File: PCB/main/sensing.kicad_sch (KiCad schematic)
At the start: 4 parts, among them U4 TO-92_Temperature_Sensor, U5 C94049_Barometer

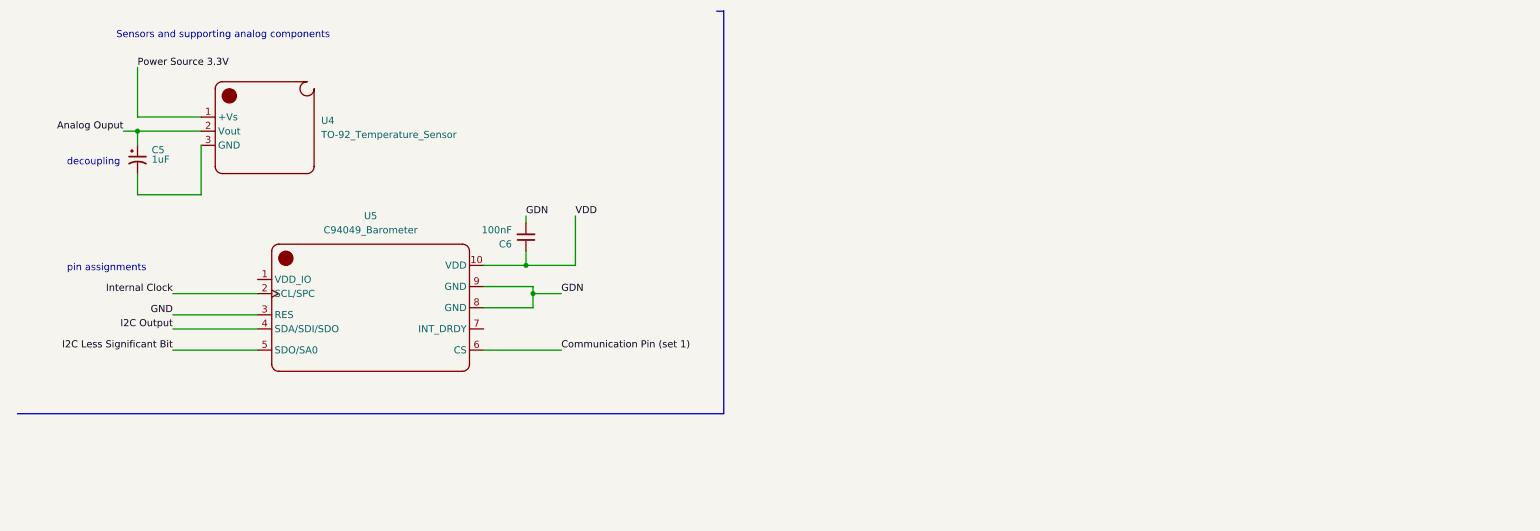
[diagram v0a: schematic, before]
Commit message: Finished initial design
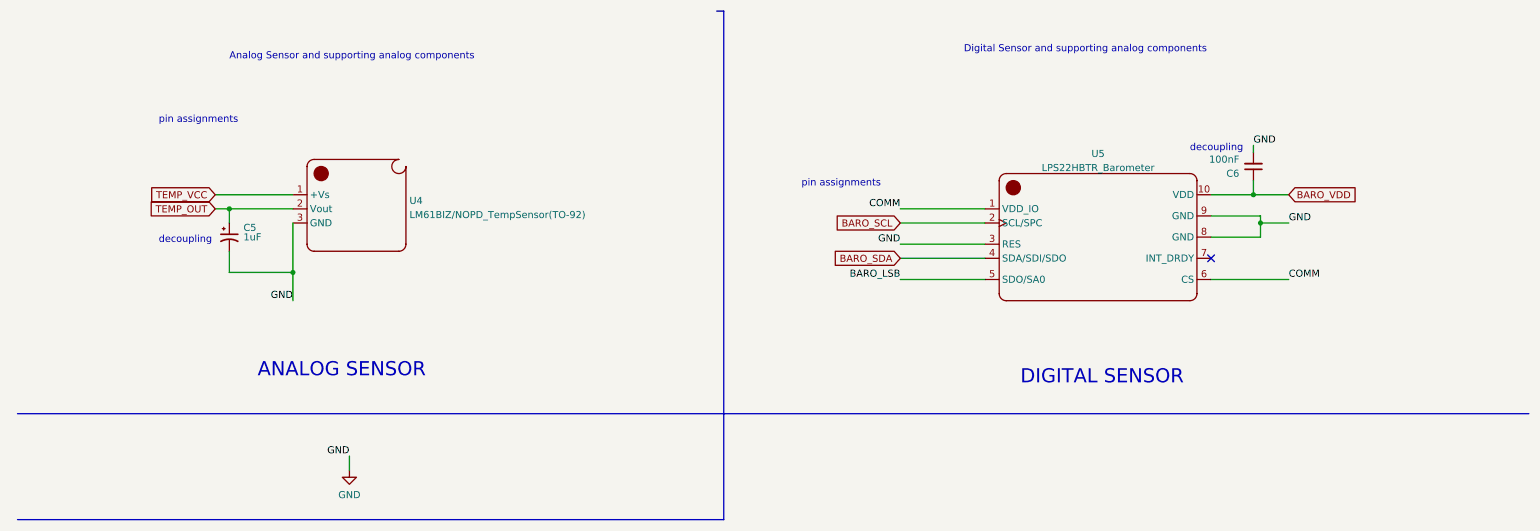
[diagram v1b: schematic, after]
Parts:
- U4: value TO-92_Temperature_Sensor -> LM61BIZ/NOPD_TempSensor(TO-92)
- U5: value C94049_Barometer -> LPS22HBTR_Barometer
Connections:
- net Communication Pin (set 1) is gone; now on net COMM: U5.6 (CS)
- net GDN is gone; now on net GND: C6.2, U5.8 (GND), U5.9 (GND)
- net GND: now also C5.2, U4.3 (GND)
- net COMM: now reaches U5.1 (VDD_IO)
- net Analog Ouput renamed TEMP_OUT
- net I2C Less Significant Bit renamed BARO_LSB
- net I2C Output renamed BARO_SDA
- net Internal Clock renamed BARO_SCL
- net Power Source 3.3V renamed TEMP_VCC
- net VDD renamed BARO_VDD
- no-connect marks 0 -> 1
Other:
- note added: "ANALOG SENSOR"
- note added: "Analog Sensor and supporting analog components"
- note added: "DIGITAL SENSOR"
- note added: "Digital Sensor and supporting analog components"
- note removed: "Sensors and supporting analog components"
- company: (none) -> University of Cape Town
- title: (none) -> Sensing Subsystem
- moved on the sheet: C5, C6, U4, U5
